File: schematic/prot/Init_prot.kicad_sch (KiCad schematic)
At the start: 34 parts, among them J1 Load, J2 Contactor, J3 FCU, J4 Conn_01x06_Pin, Q1 AO3400A, SW1 SW_DIP_x01, SW2 SW_DIP_x01, U1 STM32F070F6Px, U2 MPU-6050, U3 TPS54302

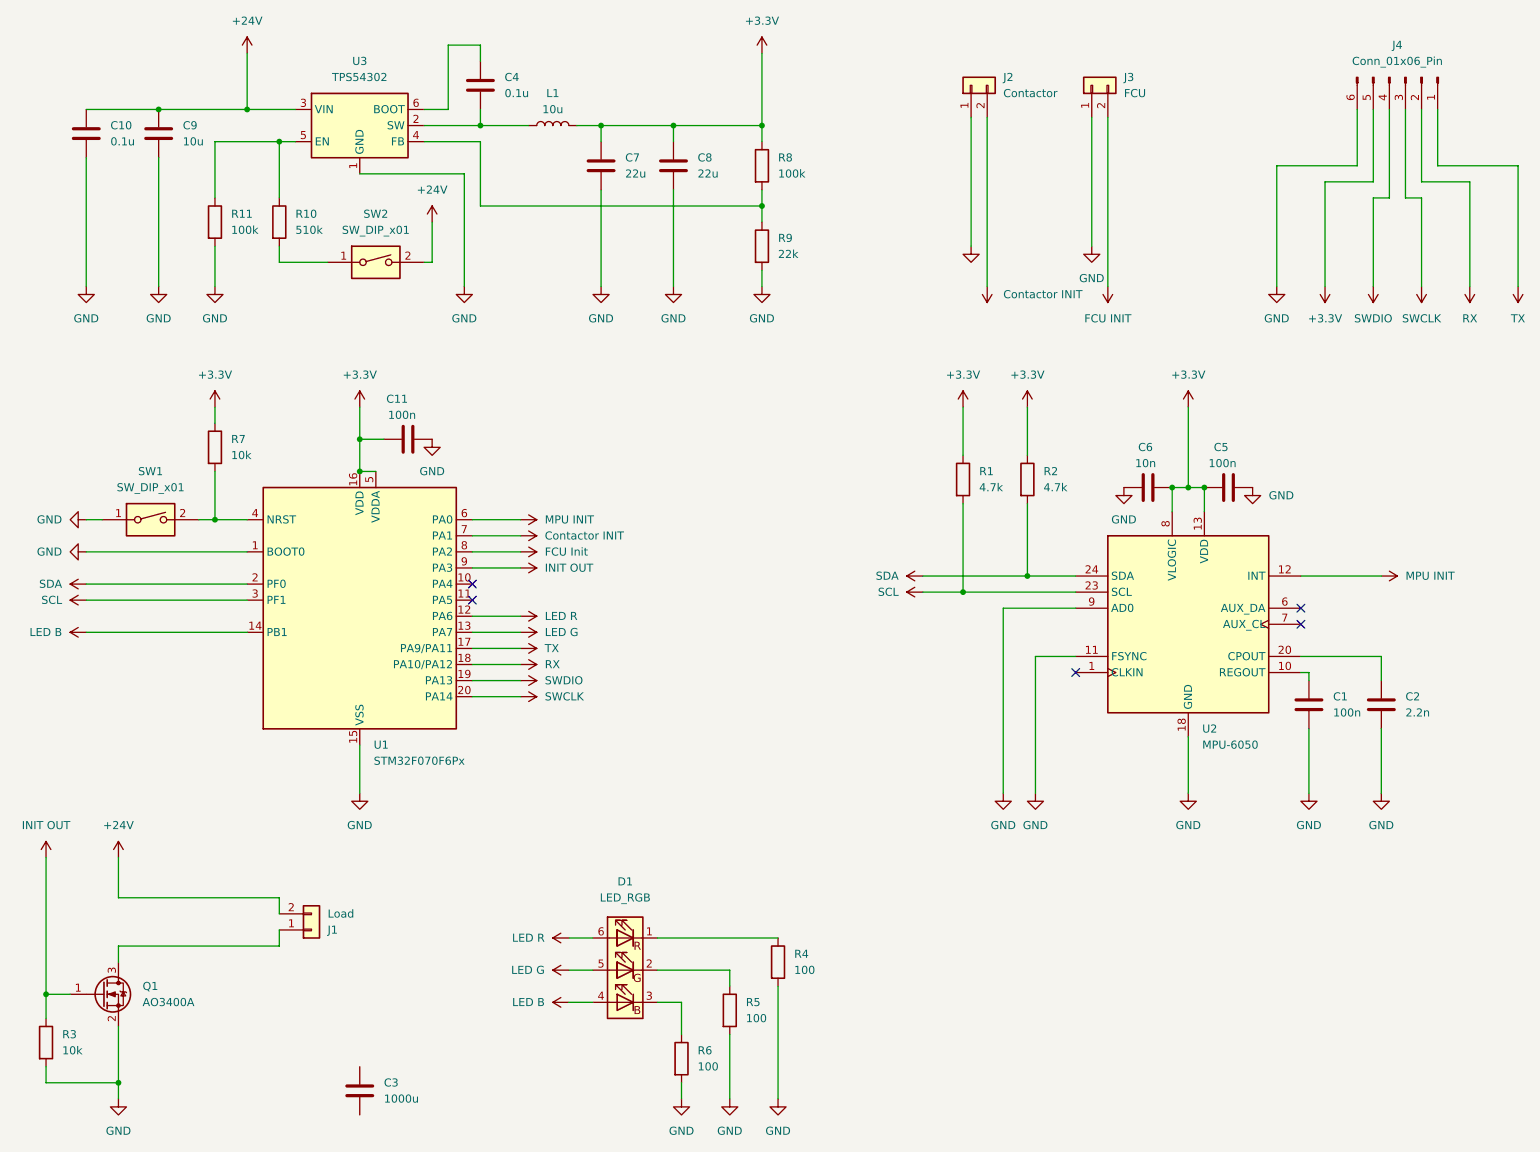
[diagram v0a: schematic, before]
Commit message: Schematic
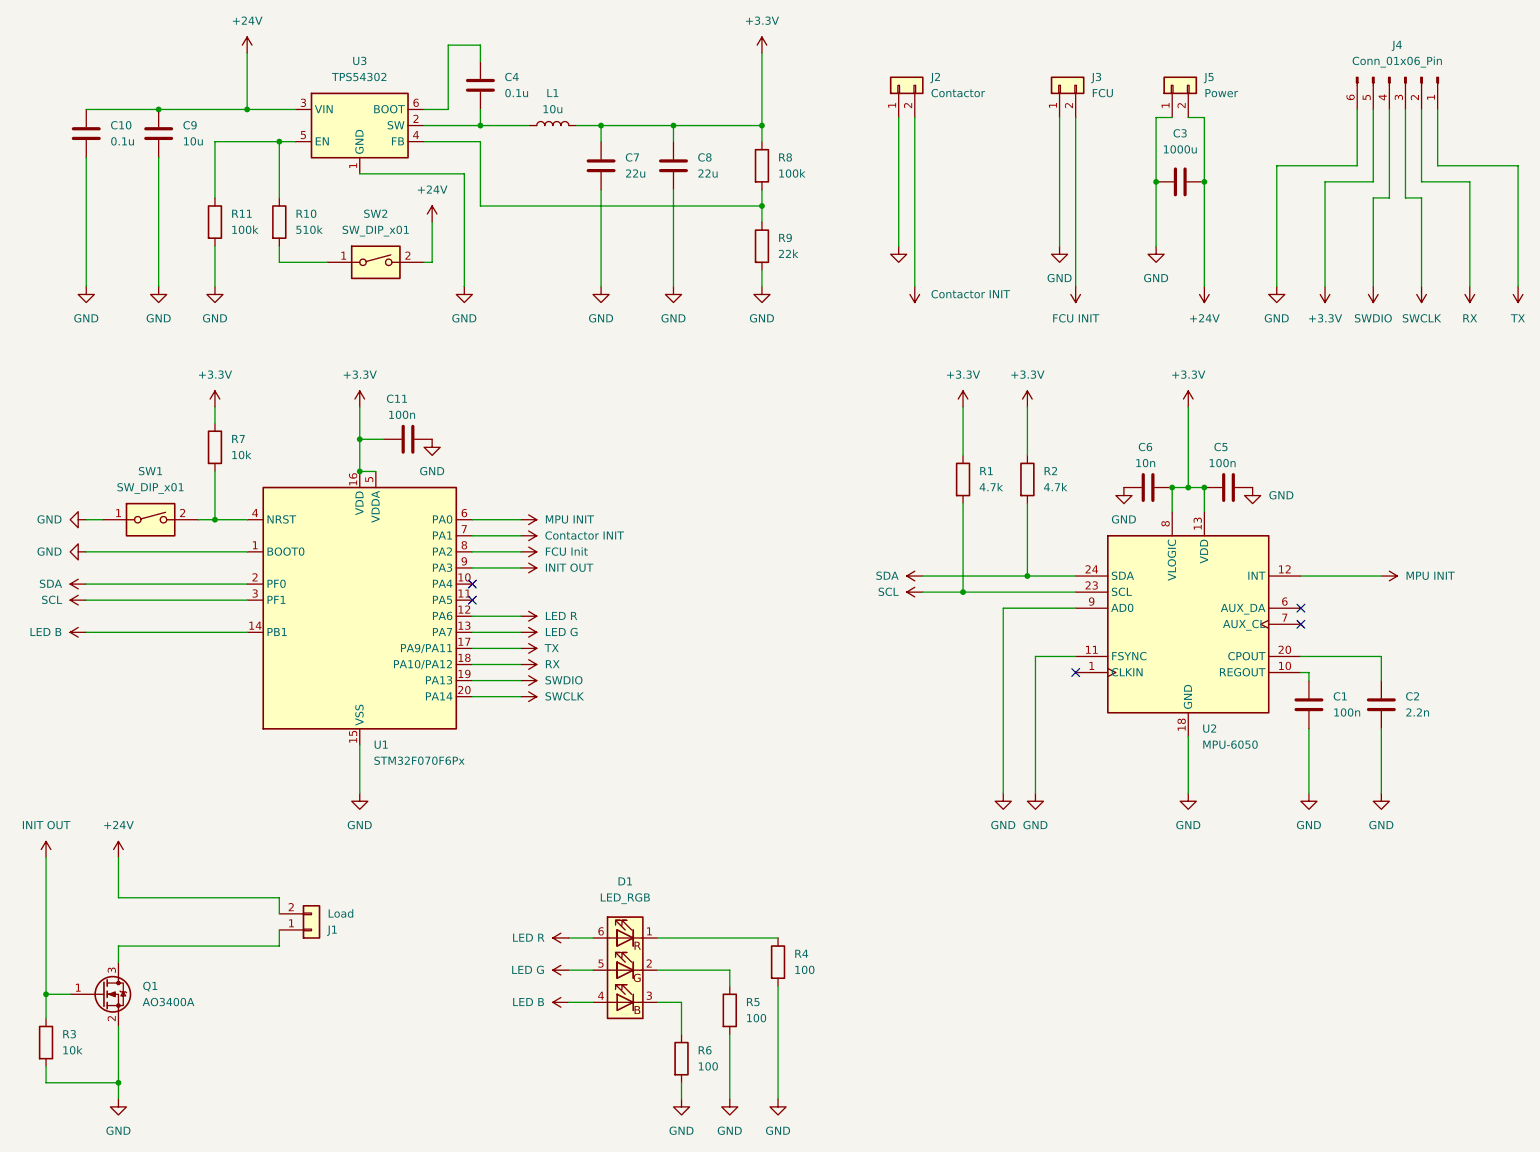
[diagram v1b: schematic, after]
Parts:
- added J5: Power, Connector_Wire:SolderWire-0.25sqmm_1x02_P4.5mm_D0.65mm_OD2mm, symbol Connector_Generic:Conn_01x02
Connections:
- net +24V: now also C3.2, J5.2 (Pin_2)
- net GND: now also C3.1, J5.1 (Pin_1)
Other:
- moved on the sheet: C3, J2, J3
